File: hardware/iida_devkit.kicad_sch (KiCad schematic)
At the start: 4 parts

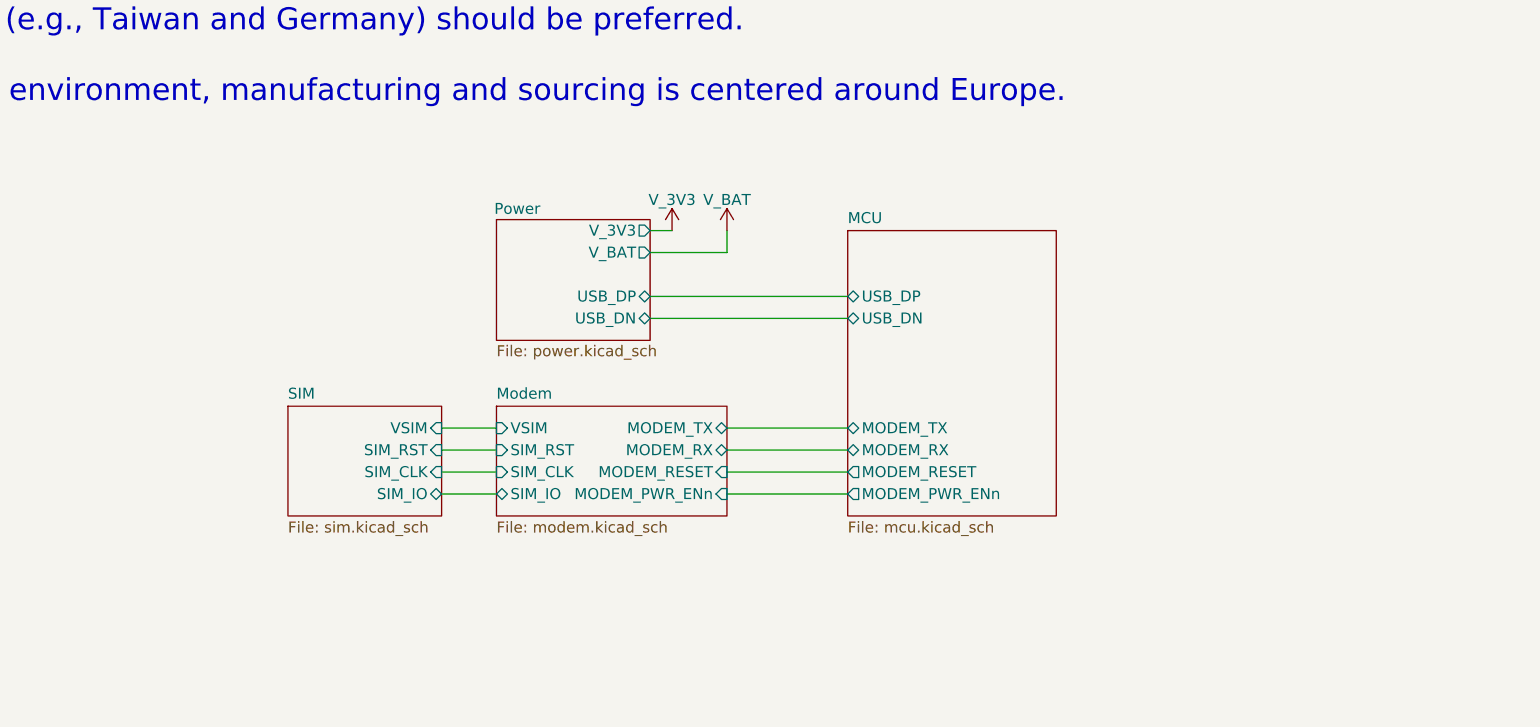
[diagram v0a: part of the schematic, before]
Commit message: HW: Start working on Hw v5.0.0
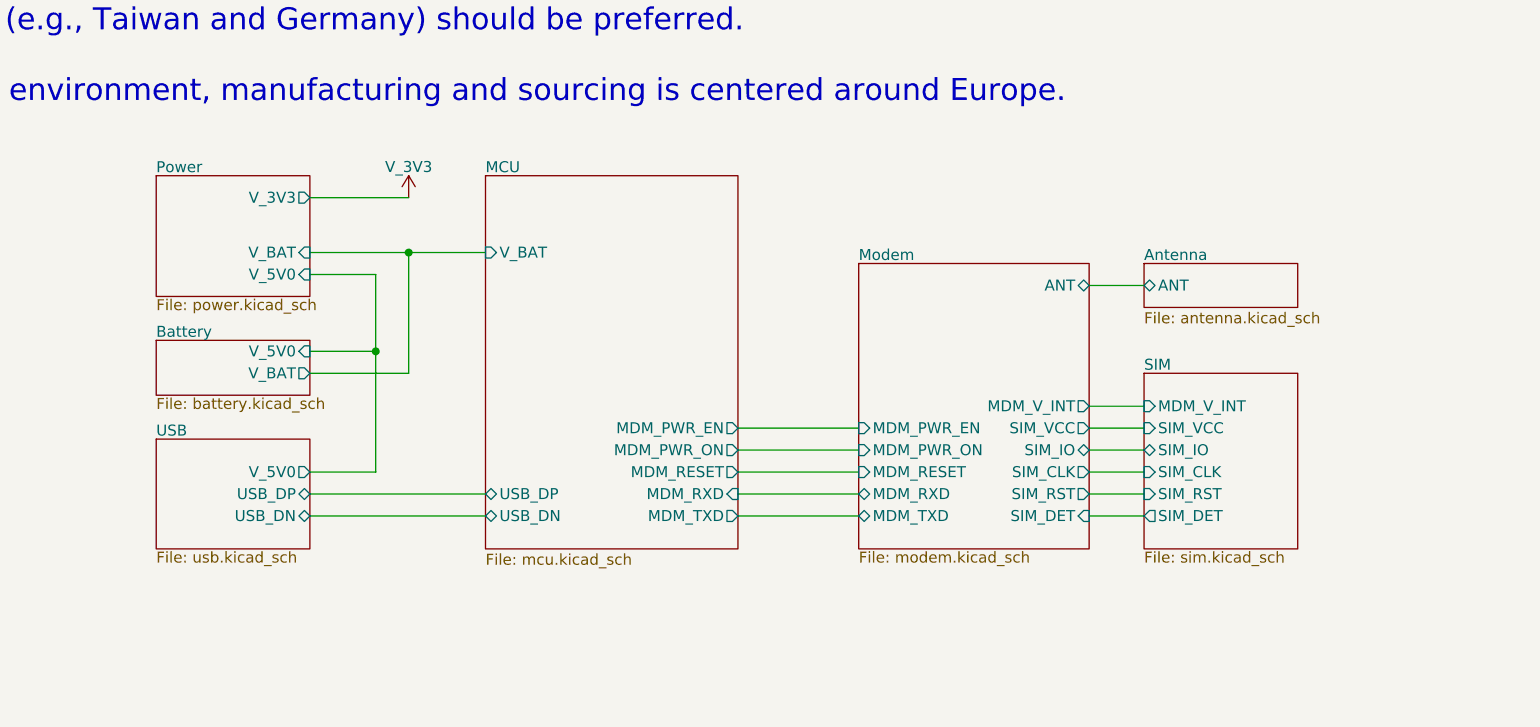
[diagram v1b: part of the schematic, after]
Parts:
- H1, H2, H3, H4: Digi-Key Part Number - -> (none)
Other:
- added sheet Antenna (antenna.kicad_sch)
- added sheet Battery (battery.kicad_sch)
- added sheet USB (usb.kicad_sch)
- sheet MCU ports: added MDM_PWR_EN, MDM_PWR_ON, MDM_RESET, MDM_RXD, MDM_TXD, V_BAT; removed MODEM_PWR_ENn, MODEM_RESET, MODEM_RX, MODEM_TX
- sheet Modem ports: added ANT, MDM_PWR_EN, MDM_PWR_ON, MDM_RESET, MDM_RXD, MDM_TXD, MDM_V_INT, SIM_DET, SIM_VCC; removed MODEM_PWR_ENn, MODEM_RESET, MODEM_RX, MODEM_TX, VSIM
- sheet Power ports: added V_5V0; removed USB_DN, USB_DP
- sheet SIM ports: added MDM_V_INT, SIM_DET, SIM_VCC; removed VSIM

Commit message: HW: Refine schematic
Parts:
- H1, H2, H3, H4: footprint MountingHole:MountingHole_2.2mm_M2_Pad_Via -> MountingHole:MountingHole_5.3mm_M5_Pad_Via
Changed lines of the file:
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@@
 			)
 		)
-		(property "Footprint" "MountingHole:MountingHole_2.2mm_M2_Pad_Via"
+		(property "Footprint" "MountingHole:MountingHole_5.3mm_M5_Pad_Via"
 			(at 134.62 189.23 0)
 			(effects
@@
 			)
 		)
-		(property "Footprint" "MountingHole:MountingHole_2.2mm_M2_Pad_Via"
+		(property "Footprint" "MountingHole:MountingHole_5.3mm_M5_Pad_Via"
 			(at 149.86 189.23 0)
 			(effects
@@
 			)
 		)
-		(property "Footprint" "MountingHole:MountingHole_2.2mm_M2_Pad_Via"
+		(property "Footprint" "MountingHole:MountingHole_5.3mm_M5_Pad_Via"
 			(at 139.7 189.23 0)
 			(effects
@@
 			)
 		)
-		(property "Footprint" "MountingHole:MountingHole_2.2mm_M2_Pad_Via"
+		(property "Footprint" "MountingHole:MountingHole_5.3mm_M5_Pad_Via"
 			(at 144.78 189.23 0)
 			(effects
